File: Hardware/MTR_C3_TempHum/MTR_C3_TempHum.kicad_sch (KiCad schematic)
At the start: 6 parts, among them IC1 ESP32-C3-MINI-1-H4, IC2 BQ25170DSGR, IC3 TLV76733DRVR, IC4 DHT22, J1 USB_C_Receptacle_USB2.0

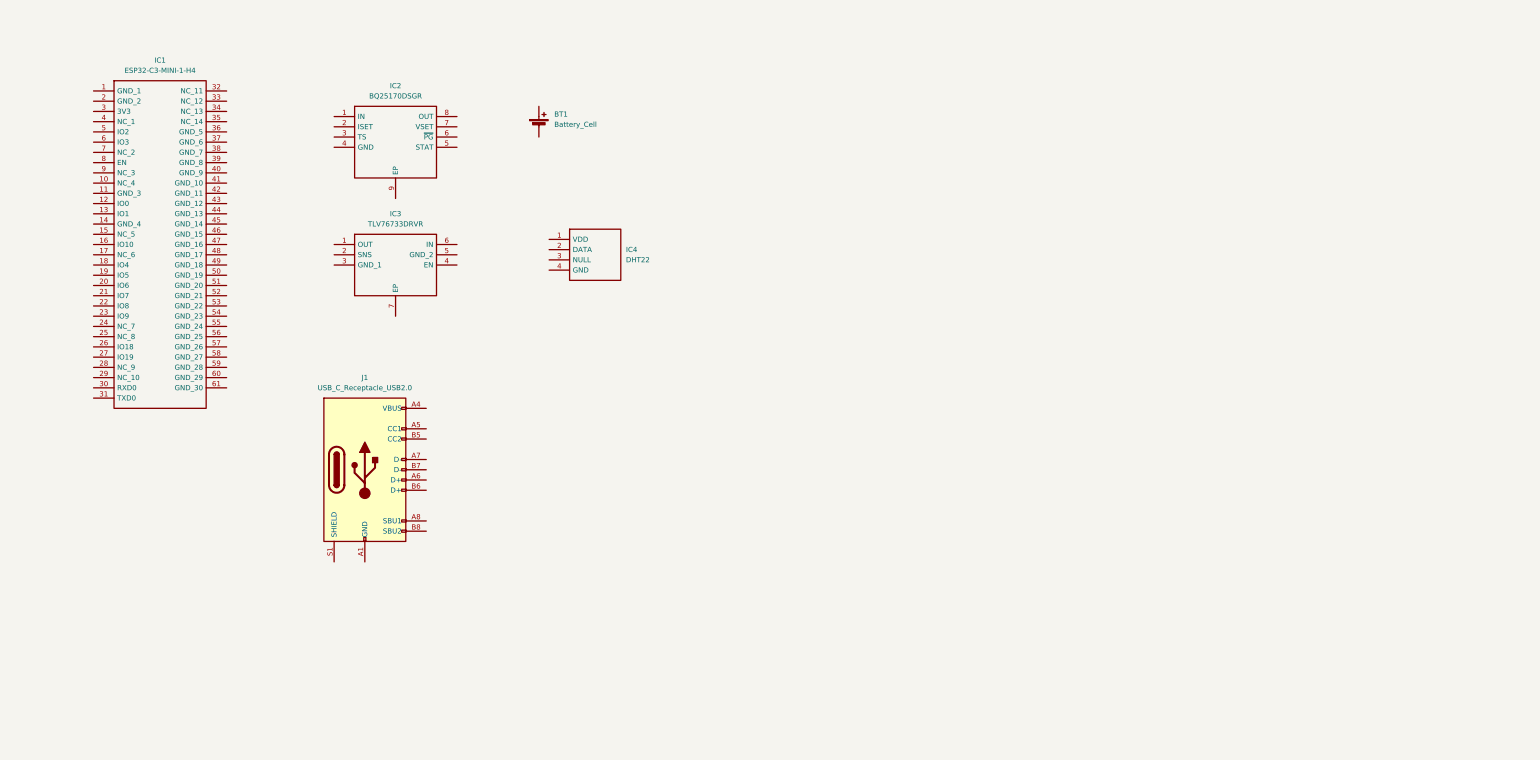
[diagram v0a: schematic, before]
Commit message: REV 0.1
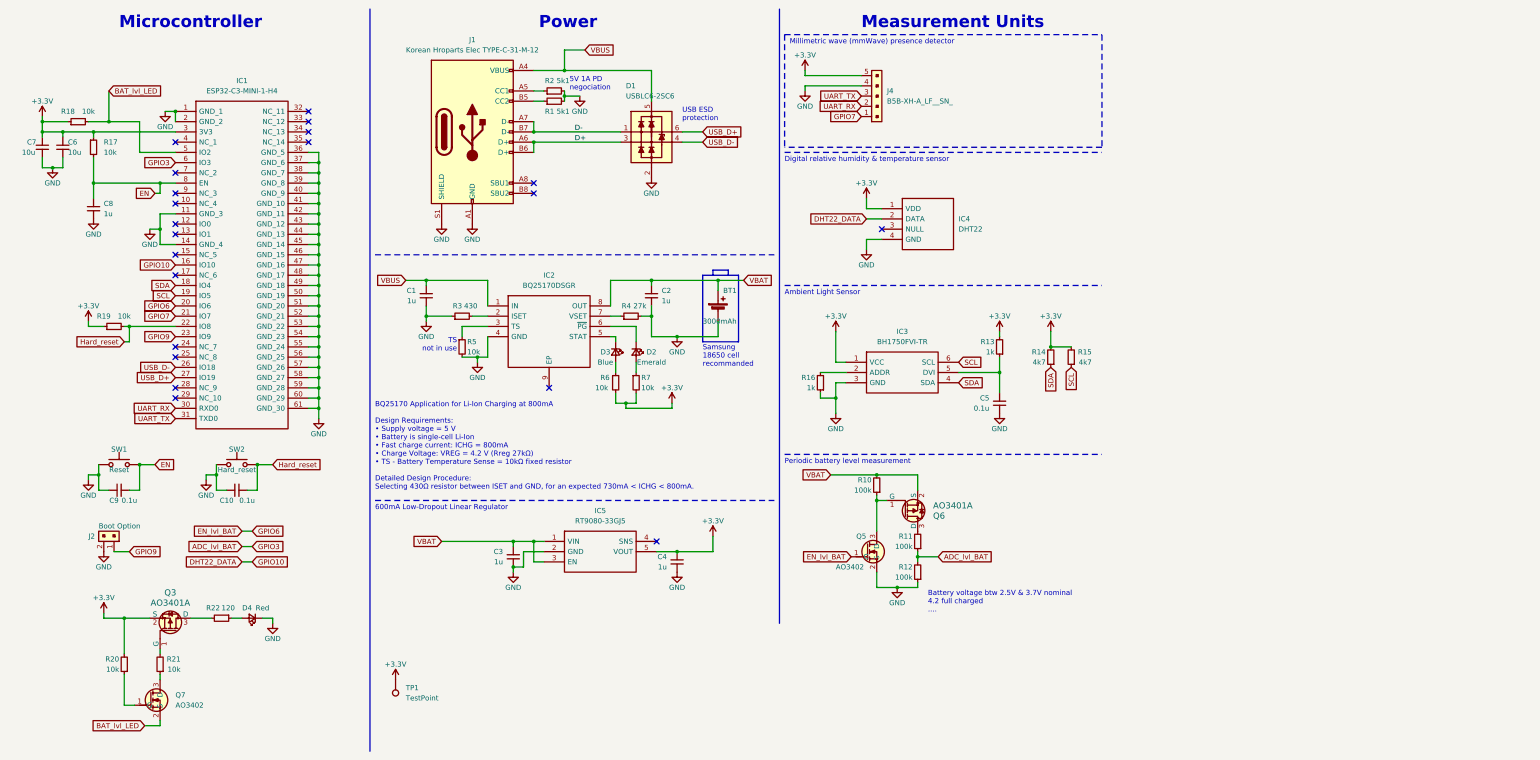
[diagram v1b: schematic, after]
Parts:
- removed IC3: TLV76733DRVR, SamacSys_Parts:SON65P200X200X80-7N, symbol SamacSys_Parts:TLV76733DRVR
- added C1, C2, C3, C4, C8: 1u, Resistor_SMD:R_0402_1005Metric, symbol Device:C_Small
- added C10, C5, C9: 0.1u, Resistor_SMD:R_0402_1005Metric, symbol Device:C_Small
- added C6, C7: 10u, Resistor_SMD:R_0402_1005Metric, symbol Device:C_Small
- added D1: USBLC6-2SC6, SamacSys_Parts:SOT95P280X145-6N, symbol PCM_Diode_TVS_AKL:USBLC6-2SC6
- added D2: Emerald, LED_SMD:LED_0603_1608Metric, symbol Device:LED_Small
- added D3: Blue, LED_SMD:LED_0603_1608Metric, symbol Device:LED_Small
- added D4: Red, LED_SMD:LED_0603_1608Metric, symbol Device:LED_Small
- added IC3: BH1750FVI-TR, SamacSys_Parts:WSOF6, symbol SamacSys_Parts:BH1750FVI-TR
- added IC5: RT9080-33GJ5, SamacSys_Parts:SOT94P280X100-5N, symbol SamacSys_Parts:RT9080-33GJ5
- added J2: Boot Option, PinHeader:PinHeader_1x02_P2.54mm_Vertical, symbol dk_Rectangular-Connectors-Headers-Male-Pins:22-23-2021
- added J4: B5B-XH-A_LF__SN_, PinHeader:PinHeader_1x05_P2.54mm_Vertical, symbol dk_Rectangular-Connectors-Headers-Male-Pins:B5B-XH-A_LF__SN_
- added Q3, Q6: AO3401A, Package_TO_SOT_SMD:SOT-23, symbol dk_Transistors-FETs-MOSFETs-Single:AO3401A
- added Q5, Q7: AO3402, Package_TO_SOT_SMD:SOT-23, symbol PCM_Transistor_MOSFET_AKL:AO3402
- added R1, R2: 5k1, Resistor_SMD:R_0402_1005Metric, symbol Device:R_Small
- added R10, R11, R12: 100k, Resistor_SMD:R_0402_1005Metric, symbol Device:R_Small
- added R13, R16: 1k, Resistor_SMD:R_0402_1005Metric, symbol Device:R_Small
- added R14, R15: 4k7, Resistor_SMD:R_0402_1005Metric, symbol Device:R_Small
- added R17, R18, R19, R20, R21, R5, R6, R7: 10k, Resistor_SMD:R_0402_1005Metric, symbol Device:R_Small
- added R22: 120, Resistor_SMD:R_0402_1005Metric, symbol Device:R_Small
- added R3: 430, Resistor_SMD:R_0402_1005Metric, symbol Device:R_Small
- added R4: 27k, Resistor_SMD:R_0402_1005Metric, symbol Device:R_Small
- added SW1: Reset, easyeda2kicad:SW-SMD_L4.0-W3.0-LS5.0, symbol Switch:SW_Push
- added SW2: Hard_reset, easyeda2kicad:SW-SMD_L4.0-W3.0-LS5.0, symbol Switch:SW_Push
- added TP1: TestPoint, TestPoint:TestPoint_Pad_D1.0mm, symbol Connector:TestPoint
- BT1: value Battery_Cell -> 3000mAh; footprint Battery:BatteryHolder_Keystone_2466_1xAAA -> easyeda2kicad:BATTERY-SMD_18650-1S-L77.1-W20.7-1; LCSC (none) -> C2988620
- IC1: LCSC (none) -> C2934569
- IC2: footprint SON50P200X200X80-9N -> SamacSys_Parts:SON50P200X200X80-9N; LCSC (none) -> C5208201
- J1: value USB_C_Receptacle_USB2.0 -> Korean Hroparts Elec TYPE-C-31-M-12; LCSC (none) -> C165948
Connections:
- net GND: now reaches IC1.1 (GND_1)
- net GND: now also BT1.2 (-), IC1.11 (GND_3), IC1.14 (GND_4), IC1.2 (GND_2), IC1.36 (GND_5), IC1.37 (GND_6), IC1.38 (GND_7), IC1.39 (GND_8), IC1.40 (GND_9), IC1.41 (GND_10), IC1.42 (GND_11), IC1.43 (GND_12), IC1.44 (GND_13), IC1.45 (GND_14), IC1.46 (GND_15), IC1.47 (GND_16), IC1.48 (GND_17), IC1.49 (GND_18), IC1.50 (GND_19), IC1.51 (GND_20), IC1.52 (GND_21), IC1.53 (GND_22), IC1.54 (GND_23), IC1.55 (GND_24), IC1.56 (GND_25), IC1.57 (GND_26), IC1.58 (GND_27), IC1.59 (GND_28), IC1.60 (GND_29), IC1.61 (GND_30), IC2.4 (GND), IC4.4 (GND), J1.A1 (GND), J1.A12 (GND), J1.B1 (GND), J1.B12 (GND), J1.S1 (SHIELD), C1.1, C10.1, C2.2, C3.1, C4.1, C5.1, C6.2, C7.2, C8.2, C9.1, D1.2 (VN), D4.1 (K), IC3.3 (GND), IC5.2 (GND), J2.2, J4.4, Q5.2 (S), R1.2, R12.1, R16.1, R2.2, R3.1, R4.2, R5.2, SW1.1, SW2.1
- net DHT22_DATA: now reaches IC1.16 (IO10)
- net DHT22_DATA: now also IC4.2 (DATA)
- net SDA: now reaches IC1.18 (IO4)
- net SDA: now also IC3.4 (SDA), R14.1
- net SCL: now reaches IC1.19 (IO5)
- net SCL: now also IC3.6 (SCL), R15.1
- net EN_lvl_BAT: now reaches IC1.20 (IO6)
- net EN_lvl_BAT: now also Q5.1 (G)
- net GPIO7: now reaches IC1.21 (IO7)
- net GPIO7: now also J4.1
- net Hard_reset: now reaches IC1.22 (IO8)
- net Hard_reset: now also C10.2, R19.2, SW2.2
- net GPIO9: now reaches IC1.23 (IO9)
- net GPIO9: now also J2.1
- net USB_D-: now reaches IC1.26 (IO18)
- net USB_D-: now also D1.4 (L2)
- net USB_D+: now reaches IC1.27 (IO19)
- net USB_D+: now also D1.6 (L1)
- net +3.3V: now reaches IC1.3 (3V3)
- net +3.3V: now also IC4.1 (VDD), C4.2, C6.1, C7.1, IC3.1 (VCC), IC5.5 (VOUT), J4.5, Q3.2 (S), R13.2, R14.2, R15.2, R17.1, R18.1, R19.1, R20.2, R6.2, R7.2, TP1.1
- net UART_RX: now reaches IC1.30 (RXD0)
- net UART_RX: now also J4.2
- net UART_TX: now reaches IC1.31 (TXD0)
- net UART_TX: now also J4.3
- net BAT_lvl_LED: now reaches IC1.5 (IO2)
- net BAT_lvl_LED: now also Q7.2 (S), R18.2
- net ADC_lvl_BAT: now reaches IC1.6 (IO3)
- net ADC_lvl_BAT: now also R11.1, R12.2
- net EN: now reaches IC1.8 (EN)
- net EN: now also C8.1, C9.2, R17.2, SW1.2
- net VBUS: now reaches J1.A4 (VBUS), J1.A9 (VBUS), J1.B4 (VBUS), J1.B9 (VBUS)
- net VBUS: now also IC2.1 (IN), C1.2, D1.5 (VP)
- net at J1.A5 (CC1): now also R2.1
- net D+: now reaches J1.A6 (D+)
- net D+: now also J1.B6 (D+), D1.3 (L2)
- net D-: now reaches J1.A7 (D-)
- net D-: now also J1.B7 (D-), D1.1 (L1)
- net at J1.B5 (CC2): now also R1.1
- net at IC2.2 (ISET): now also R3.2
- net at IC2.3 (TS): now also R5.1
- net at IC2.5 (STAT): now also D3.1 (K)
- net at IC2.6 (~{PG}): now also D2.1 (K)
- net at IC2.7 (VSET): now also R4.1
- net VBAT: now reaches IC2.8 (OUT)
- net VBAT: now also BT1.1 (+), C2.1, C3.2, IC5.1 (VIN), IC5.3 (EN), Q6.2 (S), R10.2
- new net: Q6.3 (D), R11.2
- new net: Q3.1 (G), R21.2
- new net: Q3.3 (D), R22.2
- new net: D2.2 (A), R7.1
- new net: D4.2 (A), R22.1
- new net: Q5.3 (D), Q6.1 (G), R10.1
- new net: D3.2 (A), R6.1
- new net: IC3.2 (ADDR), R16.2
- new net: C5.2, IC3.5 (DVI), R13.1
- new net: Q7.3 (D), R21.1
- new net: Q7.1 (G), R20.1
- no-connect marks 0 -> 21
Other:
- note added: "5V 1A PD negociation"
- note added: "600mA Low-Dropout Linear Regulator"
- note added: "Ambient Light Sensor"
- note added: "BQ25170 Application for Li-Ion Charging at 800mA Design Requirements: • Supply voltage = 5 V • Battery is single-cell Li-Ion • Fast charge current: ICHG = 800mA • Charge Voltage: VREG = 4.2 V (Rreg 27kΩ) • TS - Battery Temperature Sense = 10kΩ fixed resistor Detailed Design Procedure: Selecting 430Ω resistor between ISET and GND, for an expected 730mA < ICHG < 800mA."
- note added: "Battery voltage btw 2.5V & 3.7V nominal 4.2 full charged ...."
- note added: "Digital relative humidity & temperature sensor"
- note added: "Measurement Units"
- note added: "Microcontroller"
- note added: "Millimetric wave (mmWave) presence detector"
- note added: "Periodic battery level measurement"
- note added: "Power"
- note added: "Samsung 18650 cell recommanded"
- note added: "TS not in use"
- note added: "USB ESD protection"
- title: MTR C3 TempHum -> MTR C3 TempHumLight
- moved on the sheet: BT1, IC1, IC2, IC4, J1

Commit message: V0.2.0
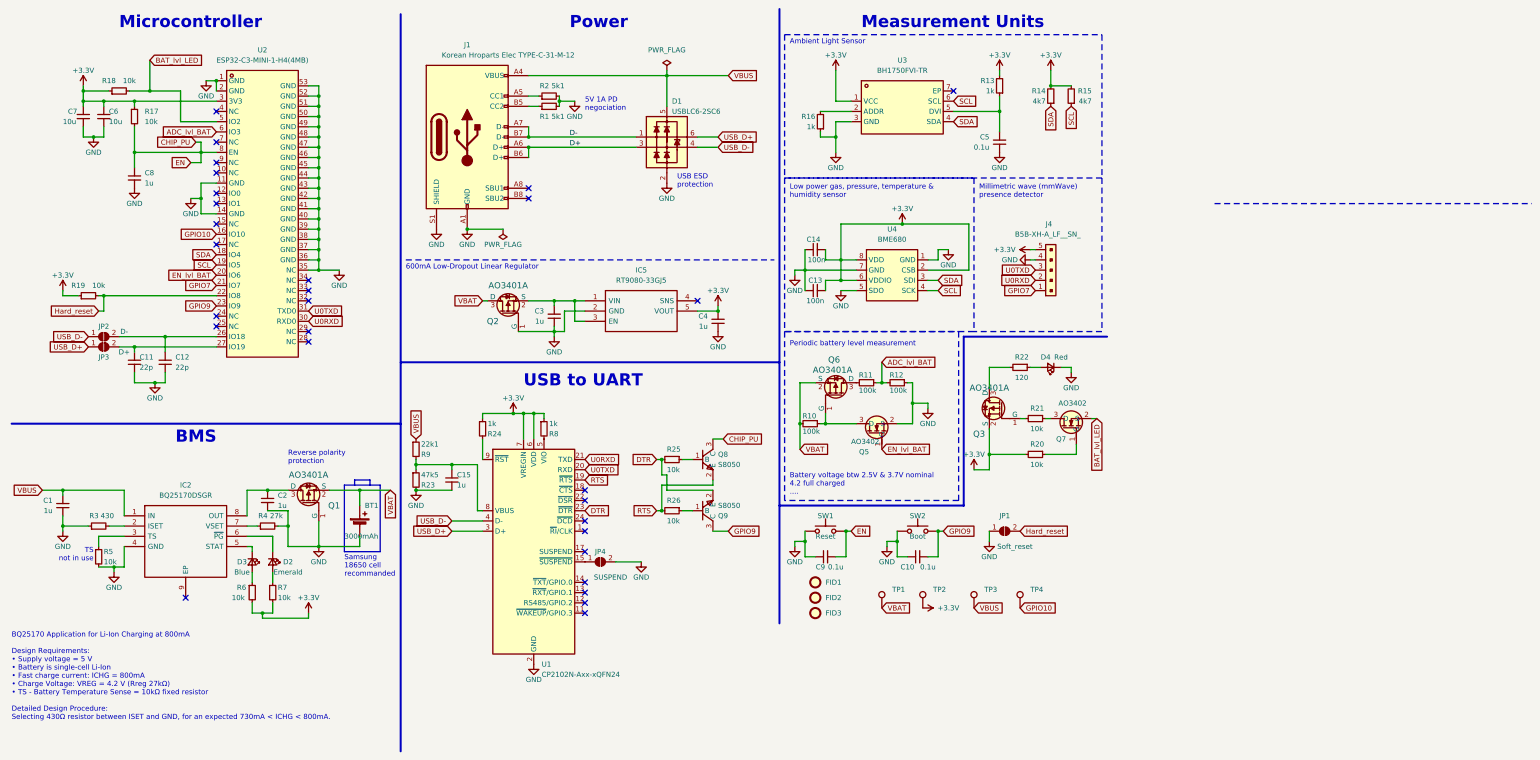
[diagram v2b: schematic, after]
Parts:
- removed IC1: ESP32-C3-MINI-1-H4, SamacSys_Parts:ESP32C3MINI1H4, symbol SamacSys_Parts:ESP32-C3-MINI-1-H4
- removed IC3: BH1750FVI-TR, SamacSys_Parts:WSOF6, symbol SamacSys_Parts:BH1750FVI-TR
- removed IC4: DHT22, SamacSys_Parts:DHT22, symbol SamacSys_Parts:DHT22
- removed J2: Boot Option, PinHeader:PinHeader_1x02_P2.54mm_Vertical, symbol dk_Rectangular-Connectors-Headers-Male-Pins:22-23-2021
- added C11, C12: 22p, Resistor_SMD:R_0402_1005Metric, symbol Device:C_Small
- added C13, C14: 100n, Resistor_SMD:R_0402_1005Metric, symbol Device:C_Small
- added C15: 1u, Resistor_SMD:R_0402_1005Metric, symbol Device:C_Small
- added FID1, FID2, FID3: Fiducial, Fiducial:Fiducial_0.75mm_Mask2.25mm, symbol Mechanical:Fiducial
- added JP1: Soft_reset, Jumper:SolderJumper-2_P1.3mm_Open_RoundedPad1.0x1.5mm, symbol Jumper:SolderJumper_2_Open
- added JP2: D-, Jumper:SolderJumper-2_P1.3mm_Open_TrianglePad1.0x1.5mm, symbol Jumper:SolderJumper_2_Open
- added JP3: D+, Jumper:jumper perso1, symbol Jumper:SolderJumper_2_Open
- added JP4: SUSPEND, Jumper:SolderJumper-2_P1.3mm_Open_TrianglePad1.0x1.5mm, symbol Jumper:SolderJumper_2_Open
- added Q1, Q2: AO3401A, Package_TO_SOT_SMD:SOT-23, symbol dk_Transistors-FETs-MOSFETs-Single:AO3401A
- added Q8, Q9: S8050, easyeda2kicad:SOT-23-3_L2.9-W1.3-P1.90-LS2.4-BR, symbol easyeda2kicad:S8050
- added R23: 47k5, Resistor_SMD:R_0402_1005Metric, symbol Device:R_Small
- added R24, R8: 1k, Resistor_SMD:R_0402_1005Metric, symbol Device:R_Small
- added R25, R26: 10k, Resistor_SMD:R_0402_1005Metric, symbol Device:R_Small
- added R9: 22k1, Resistor_SMD:R_0402_1005Metric, symbol Device:R_Small
- added TP2, TP3, TP4: TestPoint, TestPoint:TestPoint_Pad_D1.0mm, symbol Connector:TestPoint
- added U1: CP2102N-Axx-xQFN24, Package_DFN_QFN:QFN-24-1EP_4x4mm_P0.5mm_EP2.6x2.6mm, symbol Interface_USB:CP2102N-Axx-xQFN24
- added U2: ESP32-C3-MINI-1-H4(4MB), easyeda2kicad:WIFIM-SMD_ESP32-C3-MINI-1, symbol easyeda2kicad:ESP32-C3-MINI-1-H4(4MB)
- added U3: BH1750FVI-TR, easyeda2kicad:WSOF-6_L2.6-W1.6-P0.50-TL-EP, symbol easyeda2kicad:BH1750FVI-TR
- added U4: BME680, easyeda2kicad:LGA-8_L3.0-W3.0-P0.80-TR, symbol easyeda2kicad:BME680
- D1: footprint SamacSys_Parts:SOT95P280X145-6N -> easyeda2kicad:SOT-23-6_L2.9-W1.6-P0.95-LS2.8-BL
- IC2: footprint SamacSys_Parts:SON50P200X200X80-9N -> easyeda2kicad:WSON-8_L2.0-W2.0-P0.50-TL-EP
- IC5: footprint SamacSys_Parts:SOT94P280X100-5N -> easyeda2kicad:TSOT-23-5_L2.9-W1.6-P0.95-LS2.8-BL
- J4: footprint PinHeader:PinHeader_1x05_P2.54mm_Vertical -> Connector_PinSocket_1.27mm:PinSocket_1x05_P1.27mm_Vertical
- SW2: value Hard_reset -> Boot
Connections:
- net +3.3V: now also C13.2, C14.2, R24.1, R8.1, TP2.1, U1.6 (VDD), U1.7 (VREGIN), U2.3 (3V3), U3.1 (VCC), U4.2 (CSB), U4.6 (VDDIO), U4.8 (VDD); no longer TP1.1
- net ADC_lvl_BAT: now also U2.6 (IO3)
- net BAT_lvl_LED: now also U2.5 (IO2)
- net EN_lvl_BAT: now also U2.20 (IO6)
- net GND: now also C11.2, C12.2, C13.1, C14.1, C15.2, JP1.1 (A), JP4.2 (B), Q1.1 (G), Q2.1 (G), R23.2, U1.2 (GND), U1.25 (GND), U2.1 (GND), U2.11 (GND), U2.14 (GND), U2.2 (GND), U2.35 (NC), U2.36 (GND), U2.37 (GND), U2.38 (GND), U2.39 (GND), U2.40 (GND), U2.41 (GND), U2.42 (GND), U2.43 (GND), U2.44 (GND), U2.45 (GND), U2.46 (GND), U2.47 (GND), U2.48 (GND), U2.49 (GND), U2.50 (GND), U2.51 (GND), U2.52 (GND), U2.53 (GND), U3.3 (GND), U4.1 (GND), U4.5 (SDO), U4.7 (GND)
- net GPIO7: now also U2.21 (IO7)
- net GPIO9: now also C10.2, SW2.2, Q9.3 (C), U2.23 (IO9)
- net Hard_reset: now also JP1.2 (B), U2.22 (IO8); no longer C10.2, SW2.2
- net SCL: now also U2.19 (IO5), U3.6 (SCL), U4.4 (SCK)
- net SDA: now also U2.18 (IO4), U3.4 (SDA), U4.3 (SDI)
- net USB_D+: now also JP3.1 (A), U1.3 (D+)
- net USB_D-: now also JP2.1 (A), U1.4 (D-)
- net VBAT: now also TP1.1, Q1.2 (S), Q2.3 (D); no longer C2.1, C3.2, IC2.8 (OUT), IC5.1 (VIN), IC5.3 (EN)
- net VBUS: now also R9.1, TP3.1
- net at R16.2: now also U3.2 (ADDR)
- net at C5.2, R13.1: now also U3.5 (DVI)
- net EN renamed CHIP_PU
- net CHIP_PU: now also Q8.3 (C), U2.8 (EN)
- net UART_RX renamed U0RXD
- net U0RXD: now also U1.21 (TXD), U2.30 (RXD0)
- net UART_TX renamed U0TXD
- net U0TXD: now also U1.20 (RXD), U2.31 (TXD0)
- new net: C11.1, JP3.2 (B), U2.27 (IO19)
- new net: Q9.1 (B), R26.1
- new net: C3.2, IC5.1 (VIN), IC5.3 (EN), Q2.2 (S)
- new net: Q8.1 (B), R25.1
- new net: R24.2, U1.9 (~{RST})
- new net: R8.2, U1.5 (VIO)
- new net: C12.1, JP2.2 (B), U2.26 (IO18)
- new net: C15.1, R23.1, R9.2, U1.8 (VBUS)
- new net: JP4.1 (A), U1.15 (~{SUSPEND})
- new net: C2.1, IC2.8 (OUT), Q1.3 (D)
- new net DTR: Q9.2 (E), R25.2, U1.23 (~{DTR})
- new net GPIO10: TP4.1, U2.16 (IO10)
- new net RTS: Q8.2 (E), R26.2, U1.19 (~{RTS})
- no-connect marks 21 -> 29
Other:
- note added: "BMS"
- note added: "Low power gas, pressure, temperature & humidity sensor"
- note added: "Reverse polarity protection"
- note added: "USB to UART"
- note removed: "Digital relative humidity & temperature sensor"
- moved on the sheet: BT1, C1, C10, C2, C3, C4, C5, C6, C7, C8, C9, D1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

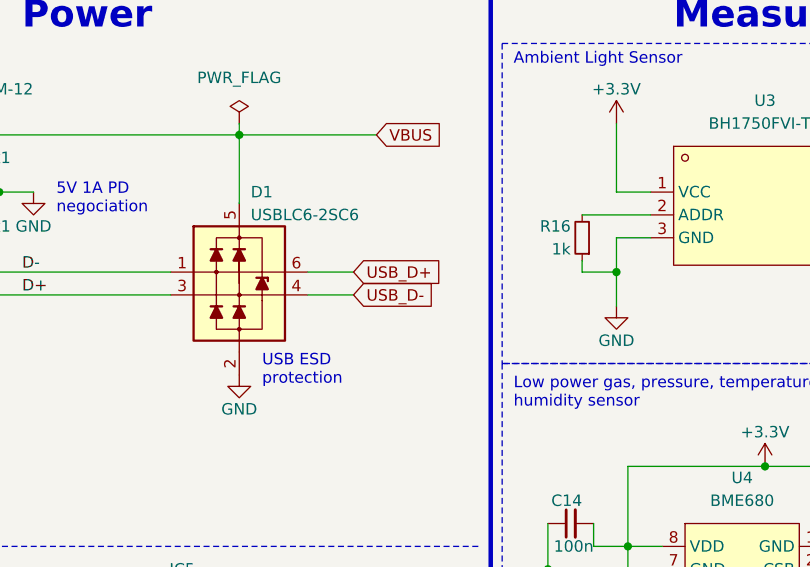
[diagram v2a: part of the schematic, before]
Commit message: ---
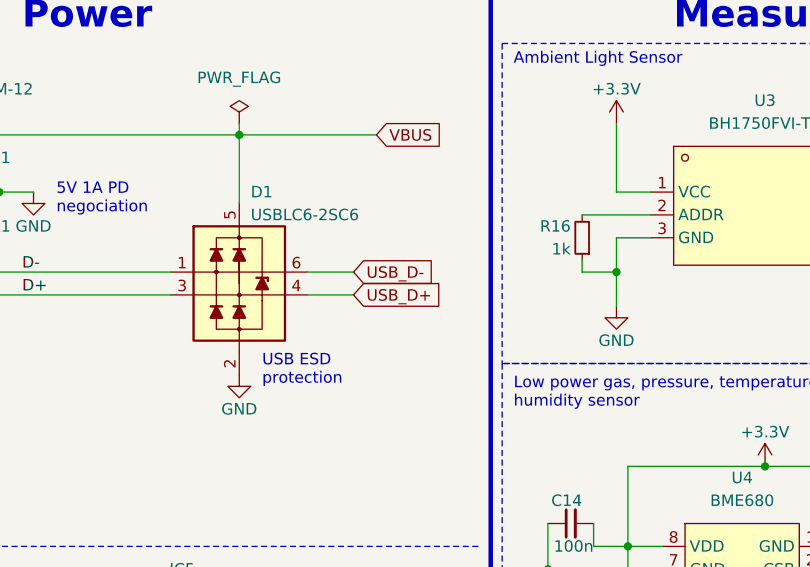
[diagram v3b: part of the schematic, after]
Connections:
- net USB_D+: now also D1.4 (L2); no longer D1.6 (L1)
- net USB_D-: now also D1.6 (L1); no longer D1.4 (L2)
